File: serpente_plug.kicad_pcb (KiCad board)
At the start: 2 copper layers, 28.8 x 22 mm, 27 parts, among them J1 USB_A, J2 Conn_Power, J3 Conn_GPIO, SW1 SW_RESET, U1 GD25Q32CNIGR, U2 MCP1700-3302E_SOT23, U3 ATSAMD21E18A

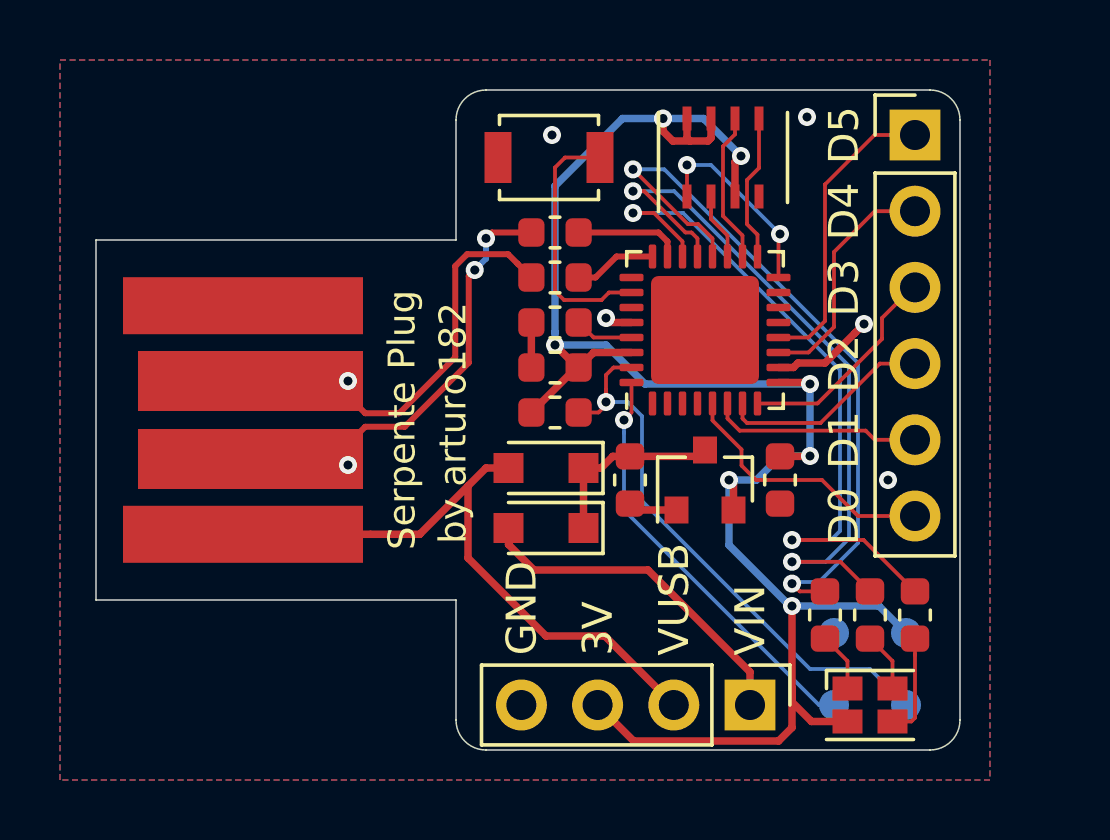
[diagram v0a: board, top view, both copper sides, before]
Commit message: Final rev 2 release!
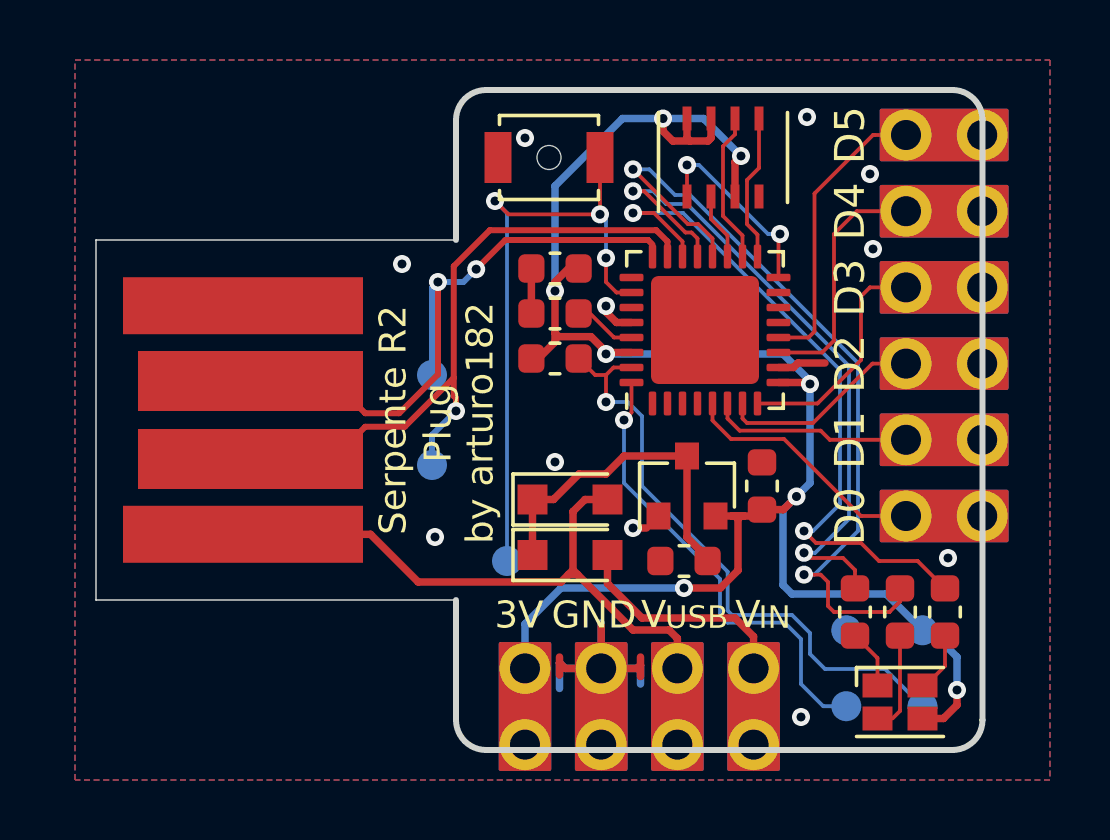
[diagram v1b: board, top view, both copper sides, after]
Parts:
- removed R7, R8: 22R, Resistor_SMD:R_0603_1608Metric
- added TP7: TP_RESET, TestPoint:TestPoint_Pad_D1.0mm, B.Cu at (125.9, 60.7)
- D3: value LED_ARGB -> LED_RBAG
- J2: footprint Connector_PinHeader_2.54mm:PinHeader_1x04_P2.54mm_Vertical -> Connector_PinHeader_2.54mm_Extra:PinHeader_1x04_P2.54mm_Vertical_Castellated
- J3: footprint Connector_PinHeader_2.54mm:PinHeader_1x06_P2.54mm_Vertical -> Connector_PinHeader_2.54mm_Extra:PinHeader_1x06_P2.54mm_Vertical_Castellated
- SW1: footprint Button_Switch_SMD:SW_SPST_B3U-1000P -> Button_Switch_SMD:SW_SPST_B3U-1000P-B
- moved TP5 4.40 mm to (123.4, 57.5)
- moved TP6 4.40 mm to (123.4, 54.5)
- moved C2 3.30 mm to (127.5, 51.0)
- moved C1 3.24 mm to (131.8, 60.7), turned to 0 degrees
- moved R3 2.50 mm to (140.5, 62.4)
- moved R6 1.80 mm to (127.5, 54.0)
- moved D1 1.32 mm to (128.0, 58.6), turned to 0 degrees
- moved J2 1.23 mm to (134.1, 64.3)
- moved D2 1.20 mm to (128.0, 60.5), turned to 0 degrees
- moved R1 1.00 mm to (137.5, 62.4)
- moved D3 1.00 mm to (139.0, 65.4)
- moved C3 0.63 mm to (134.4, 58.2), turned to 90 degrees
- moved U2 0.63 mm to (131.9, 58.2)
- moved TP3 0.56 mm to (139.8, 63.0)
- moved TP1 0.55 mm to (139.8, 65.5)
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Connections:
- net Net-(SW1-Pad2) renamed /~RESET~
- D3 pad 3: Net-(D3-Pad3) -> +3V3
- D3 pad 4: +3V3 -> Net-(D3-Pad4)
- J2 pad 3: +3V3 -> GND
- J2 pad 4: GND -> +3V3
- R2 pad 1: Net-(D3-Pad3) -> Net-(D3-Pad4)
- U3 pad 20: /LED_R -> /LED_G
- U3 pad 21: /LED_B -> /LED_R
- U3 pad 22: /LED_G -> /LED_B
- U3 pad 23: Net-(R7-Pad1) -> /USB_D-
- U3 pad 24: Net-(R8-Pad1) -> /USB_D+
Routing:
- net /~RESET~: track 8.53 -> 21.1 mm, vias 0 -> 3
- net GND: track 7.60 -> 18.5 mm, vias 5 -> 11
- net +5V: track 6.30 -> 11.3 mm
- net /LED_G: track 23.5 -> 27.1 mm
- net Net-(R7-Pad1): track 3.59 -> 0.00 mm
- net Net-(D3-Pad3): track 3.44 -> 0.00 mm
- net /GPIO4: track 7.97 -> 10.8 mm
- net Net-(D3-Pad4): track 0.00 -> 2.87 mm
- net /GPIO3: track 7.26 -> 10.1 mm
- net Net-(R8-Pad1): track 2.75 -> 0.00 mm
- net /GPIO5: track 10.0 -> 12.3 mm
- net /GPIO2: track 7.13 -> 9.39 mm
- net /GPIO1: track 7.04 -> 9.30 mm
- net VBUS: track 21.1 -> 23.2 mm
- net /GPIO0: track 8.95 -> 10.9 mm
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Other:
- board size 28.8 x 22 mm -> 29.5 x 22 mm
- board text added: "CLK"
- board text added: "DAT"
- board text added: "IN"
- board text added: "Plug"
- board text added: "RST"
- board text added: "Serpente R2"
- board text added: "USB"
- board text added: "V"
- board text removed: "C"
- board text removed: "G"
- board text removed: "JLCJLCJLCJLC"
- board text removed: "Serpente Plug"
- board text removed: "VIN"
- board text removed: "VUSB"
